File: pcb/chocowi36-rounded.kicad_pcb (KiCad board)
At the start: 2 copper layers, 113.1 x 88.3 mm, 29 parts, among them SW10 SW_Push, SW11 SW_Push, SW12 SW_Push, SW14 SW_Push, SW15 SW_Push, SW16 SW_Push, SW17 SW_Push, SW18 SW_Push, SW19 SW_Push, SW2 SW_Push, SW20 SW_Push, SW21 SW_Push, SW3 SW_Push, SW4 SW_Push, SW5 SW_Push, SW6 SW_Push, SW8 SW_Push, SW9 SW_Push, U1 nice!nano, U2 nice!nano

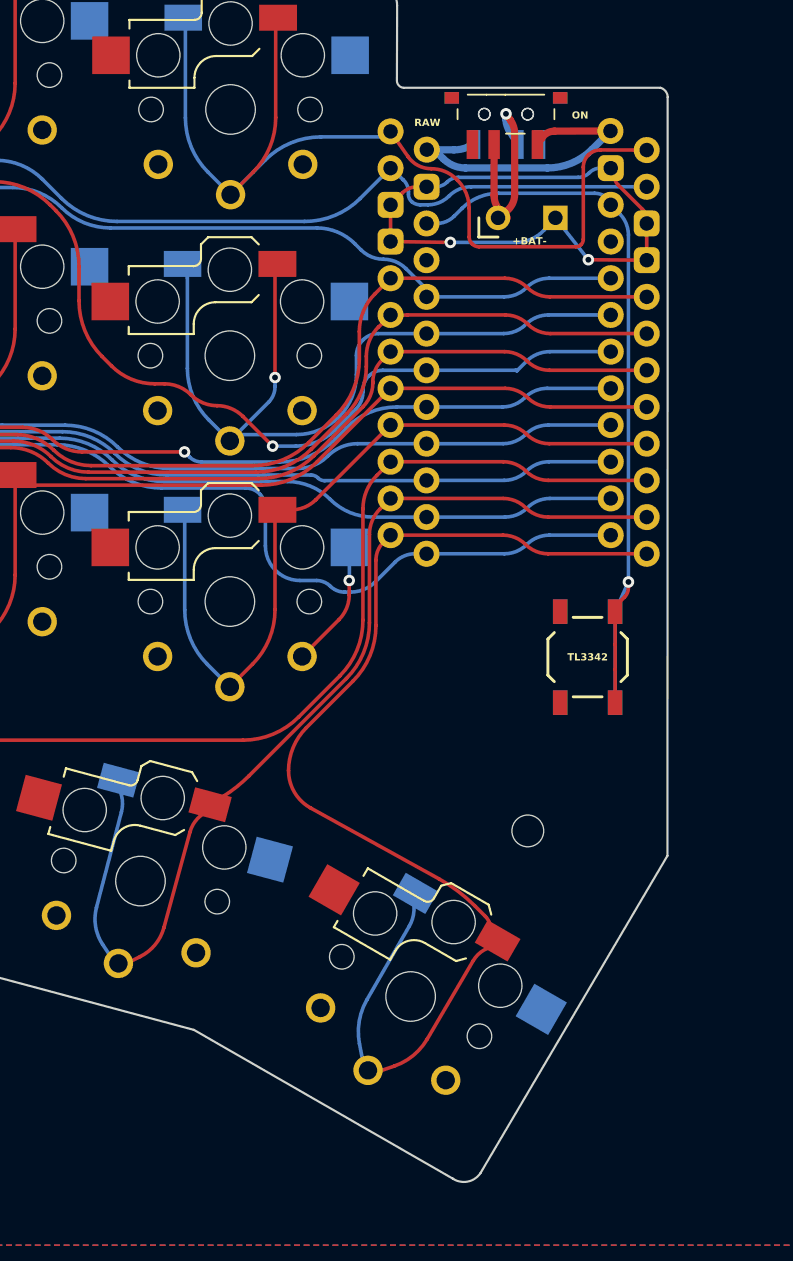
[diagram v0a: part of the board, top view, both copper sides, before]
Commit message: update gerber
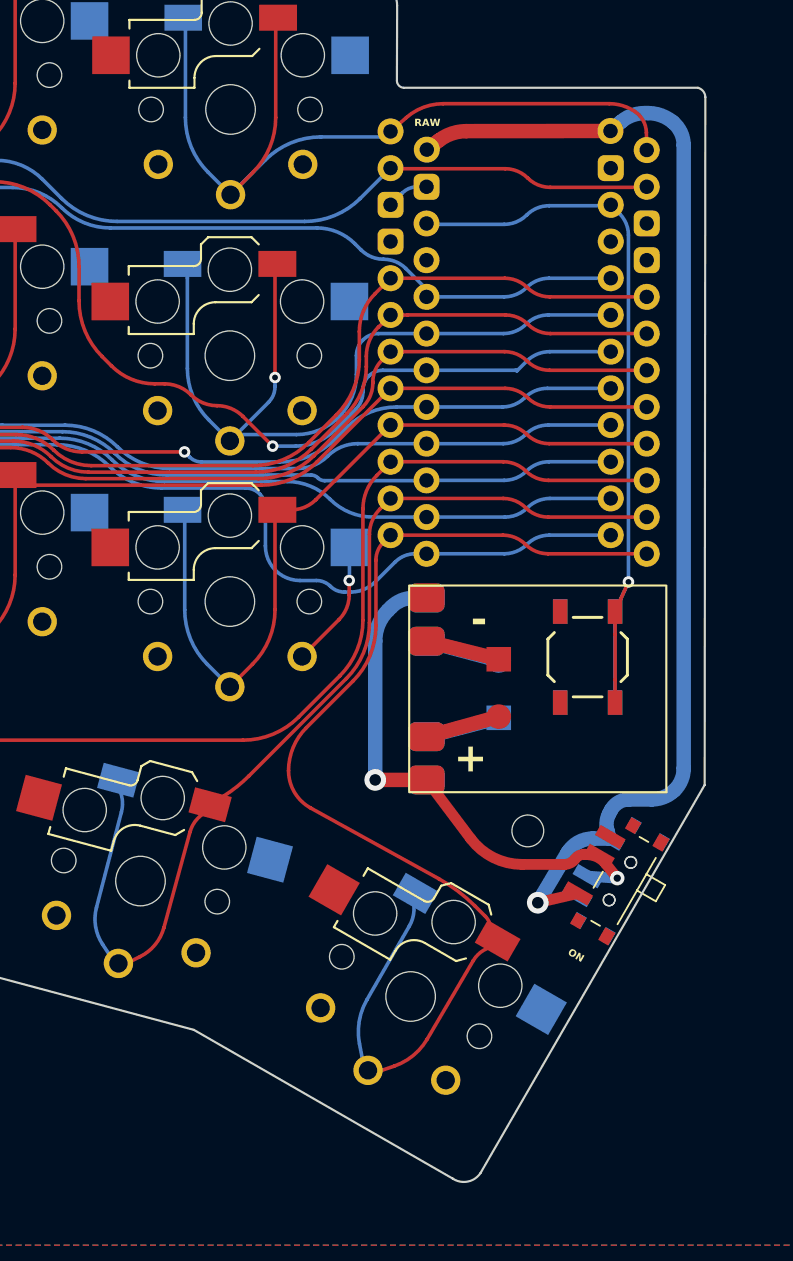
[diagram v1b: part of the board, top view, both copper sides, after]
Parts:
- added BT2: B1, itsdmd:Battery_Pads-dual-side, B.Cu at (176.6, 101.4)
- added T1: ~, itsdmd:Module_TP4056_Mini-SMD_Interface, F.Cu at (179.2, 101.5)
- added T2: ~, itsdmd:Module_TP4056_Mini-SMD_Interface, B.Cu at (179.2, 101.5)
- BT1: value Battery_Cell -> B1
- moved SW_POWER1 53.8 mm to (184.8, 115.0), turned to 60 degrees
- moved SW_POWER2 53.6 mm to (185.0, 114.7), turned to -120 degrees
- moved BT1 32.7 mm to (176.6, 101.5), turned to 90 degrees
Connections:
- BT1 pad 2: gnd -> Net-(BT1--)
- SW_POWER1 pad COM: Net-(BT1-+) -> Net-(T1-Load+)
- SW_POWER2 pad COM: Net-(BT1-+) -> Net-(T1-Load+)
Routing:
- net +BATT: track 22.3 -> 81.5 mm, vias 0 -> 1
- net gnd: track 55.0 -> 12.7 mm, vias 3 -> 1
- net Net-(T1-Load+): track 0.00 -> 37.2 mm, vias 0 -> 2
- net Net-(BT1-+): track 15.5 -> 5.19 mm, vias 1 -> 0
- net Switch6: track 68.0 -> 59.8 mm
- net Net-(BT2-+): track 0.00 -> 5.18 mm
- net Net-(BT2--): track 0.00 -> 5.17 mm
- net Net-(BT1--): track 0.00 -> 5.15 mm
- net Switch5: track 77.4 -> 76.4 mm
- net reset: track 57.4 -> 56.7 mm
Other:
- board size 113.1 x 88.3 mm -> 115.7 x 88.3 mm
- board text removed: "+BAT-"
- board text removed: "-BAT+"
